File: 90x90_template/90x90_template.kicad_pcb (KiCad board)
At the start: 2 copper layers, 90 x 90 mm, 41 parts, among them J1 Screw_Terminal_01x02

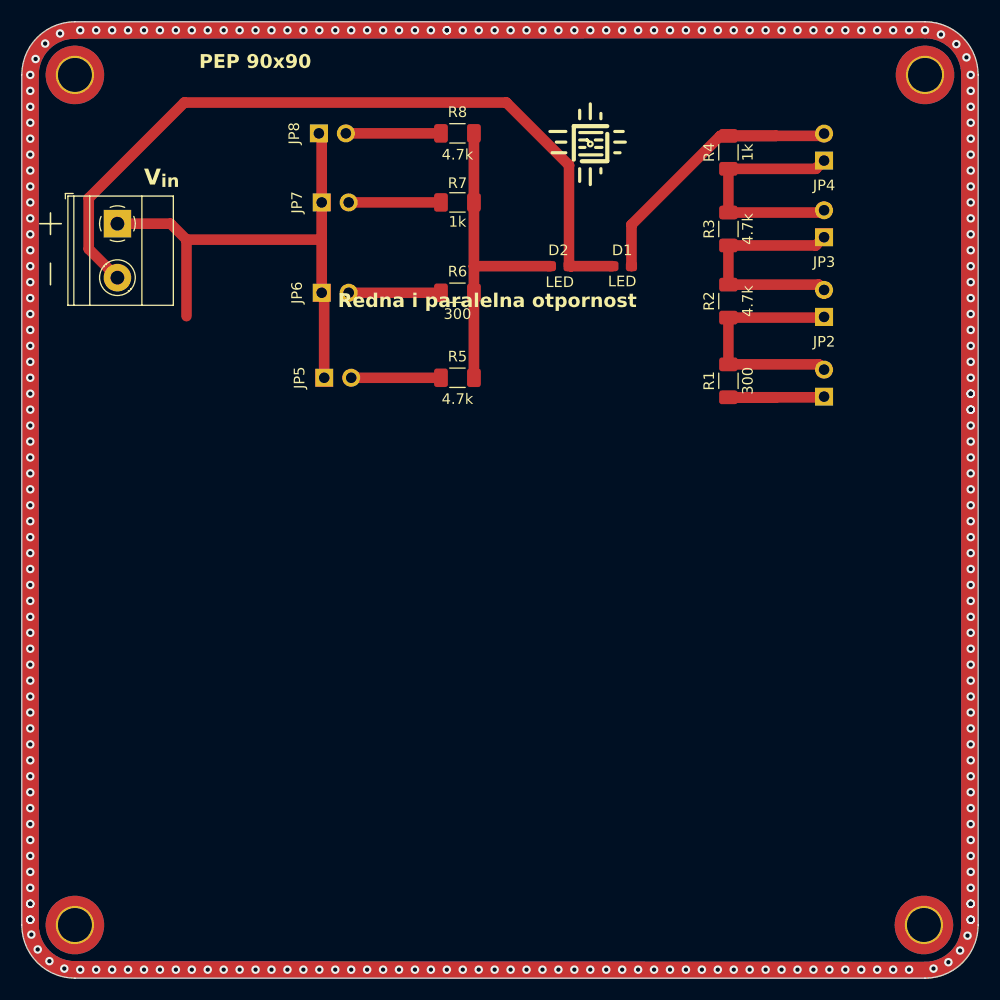
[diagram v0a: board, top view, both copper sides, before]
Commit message: Edge vias 0.
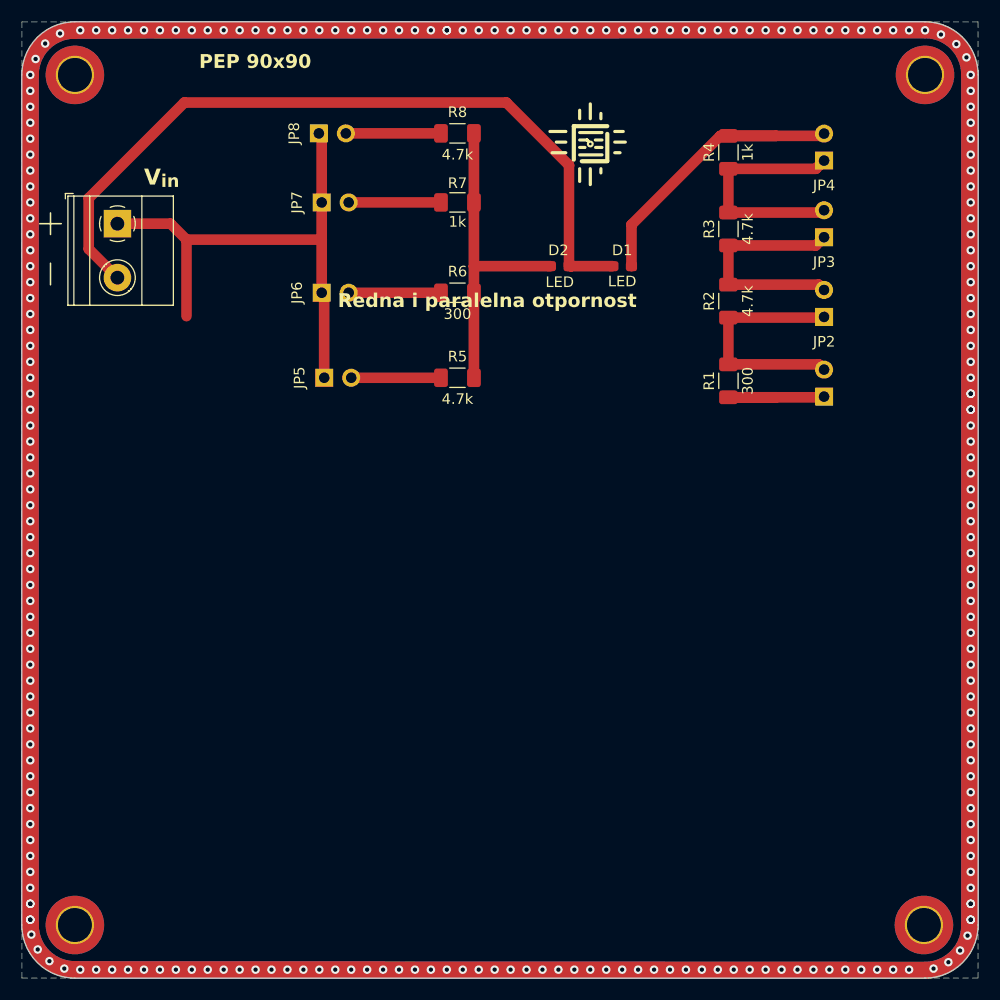
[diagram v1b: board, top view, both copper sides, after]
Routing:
- added copper zone on B.Cu, net 0
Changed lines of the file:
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@@
 		(net 11)
+	)
+	(zone
+		(net 1)
+		(net_name "0")
+		(layer "B.Cu")
+		(hatch edge 0.5)
+		(connect_pads
+			(clearance 0.5)
+		)
+		(min_thickness 0.25)
+		(filled_areas_thickness no)
+		(fill yes
+			(thermal_gap 0.5)
+			(thermal_bridge_width 0.5)
+		)
+		(polygon
+			(pts
+				(xy 100 50) (xy 190 50) (xy 190 140) (xy 100 140)
+			)
+		)
 	)
 	(embedded_fonts no)
